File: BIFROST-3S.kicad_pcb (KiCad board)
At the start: 2 copper layers, 54 x 36 mm, 14 parts, among them J1 B6B-XH-A_LF__SN_, J2 560020-1020, J3 B4B-XH-A_LF__SN_, J4 XT30PW-M, J5 XT30PW-M

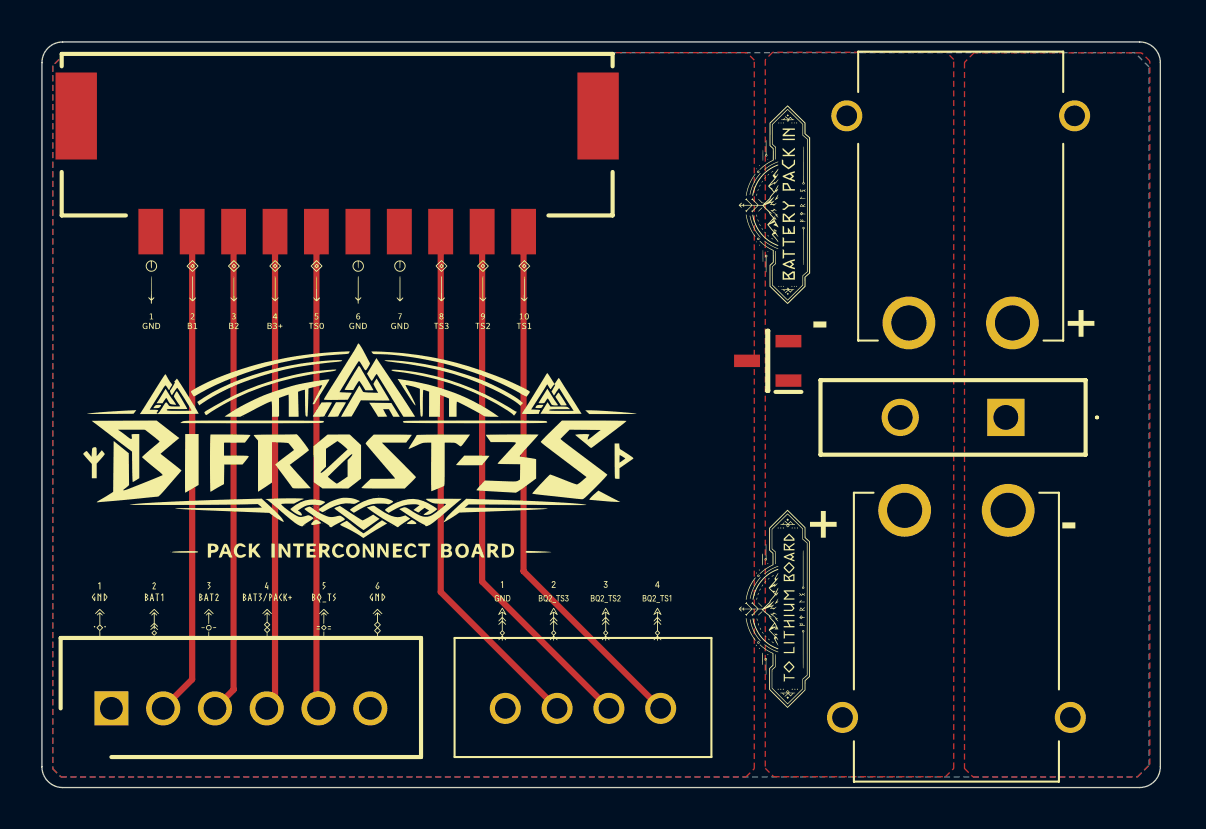
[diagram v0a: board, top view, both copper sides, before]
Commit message: Layout 4.0
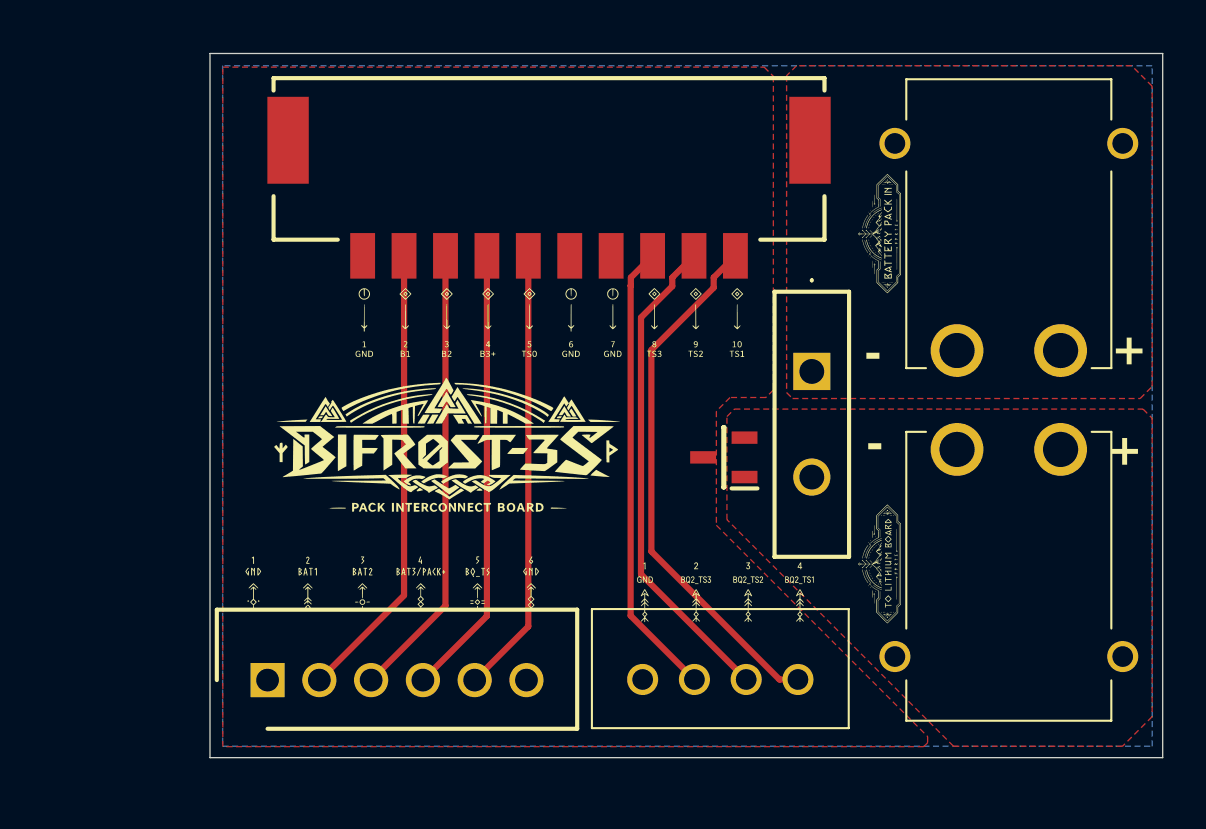
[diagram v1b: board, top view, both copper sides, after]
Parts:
- removed the G*** at (150.4, 94.5)
- removed the G*** at (130.2, 108.0)
- removed the G*** at (150.1, 114.1)
- removed the G*** at (141.7, 104.7)
- added G***: LOGO, LOGO, F.Cu at (155.3, 95.9)
- added G***: LOGO, LOGO, F.Cu at (134.4, 107.1)
- added G***: LOGO, LOGO, F.Cu at (155.2, 111.9)
- added G***: LOGO, LOGO, B.Cu at (145.8, 104.3)
- moved G*** 10.4 mm to (139.4, 100.1)
- moved J2 10.3 mm to (139.1, 92.3)
- moved F1 9.63 mm to (151.8, 102.6), turned to -90 degrees
- moved J1 7.66 mm to (125.5, 117.5)
- moved G*** 7.52 mm to (131.6, 112.8)
- moved G*** 6.94 mm to (147.5, 113.3)
- moved J3 6.78 mm to (143.7, 117.5)
- moved D1 5.12 mm to (147.6, 106.7)
- moved J4 3.88 mm to (161.3, 112.3)
- moved J5 2.68 mm to (161.3, 95.7)
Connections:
- J4 pad 1: GND -> /+BATT
- J4 pad 2: /+BATT -> GND
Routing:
- net /BQ2_TS3: track 25.3 -> 22.2 mm
- net /BQ2_TS2: track 25.6 -> 23.6 mm
- net /BQ_TS: track 23.1 -> 21.6 mm
- net /BAT3/PACK+: track 23.2 -> 21.8 mm
- net /BAT2: track 23.4 -> 22.0 mm
- net /BAT1: track 23.6 -> 22.2 mm
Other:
- board size 54 x 36 mm -> 46 x 34 mm
